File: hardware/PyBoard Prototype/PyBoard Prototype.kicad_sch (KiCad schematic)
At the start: 10 parts, among them J1 MIDI In, J2 MIDI Out, Q1 Q_PNP_BCE, U1 PyBoard_v1.1, U2 PC817, U3 MIKROE-506

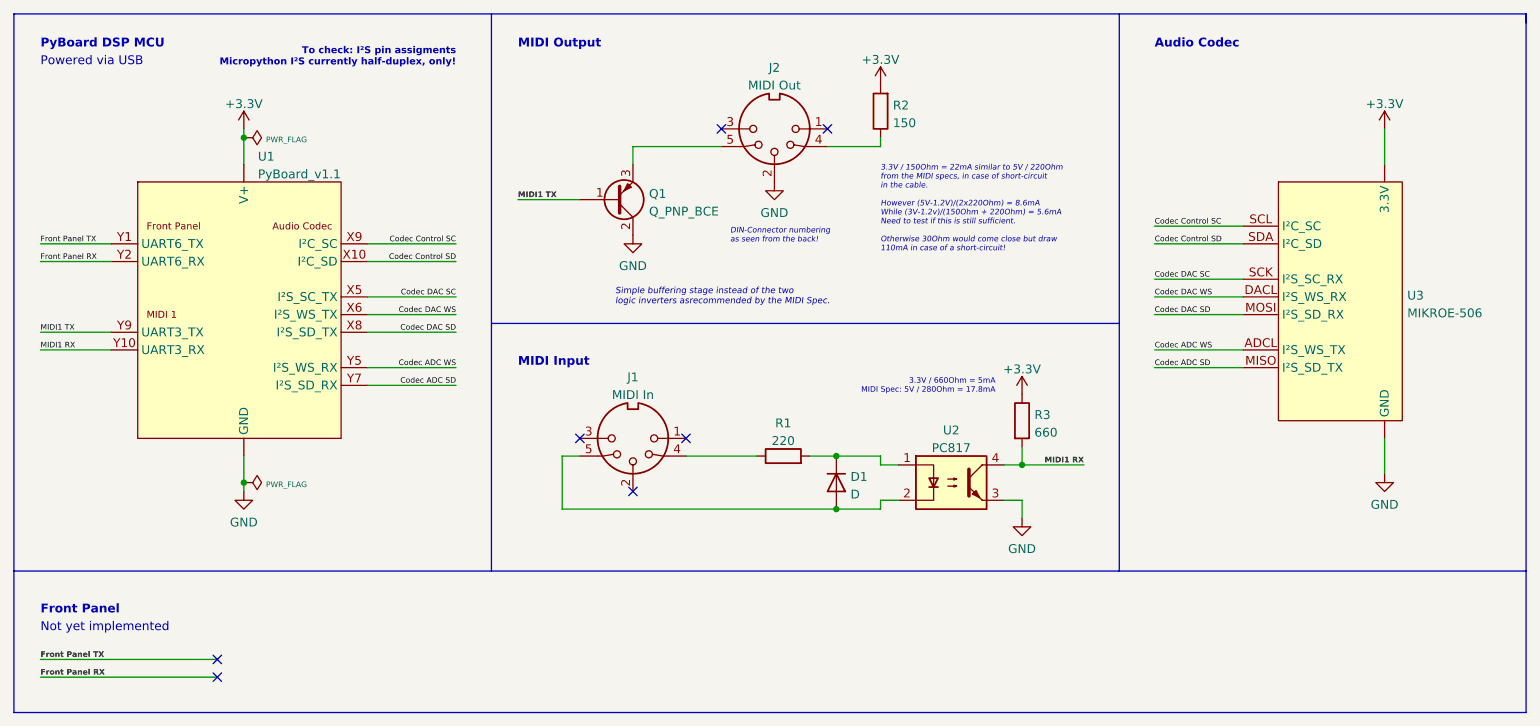
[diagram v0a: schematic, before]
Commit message: Some more experiments with MicroPython
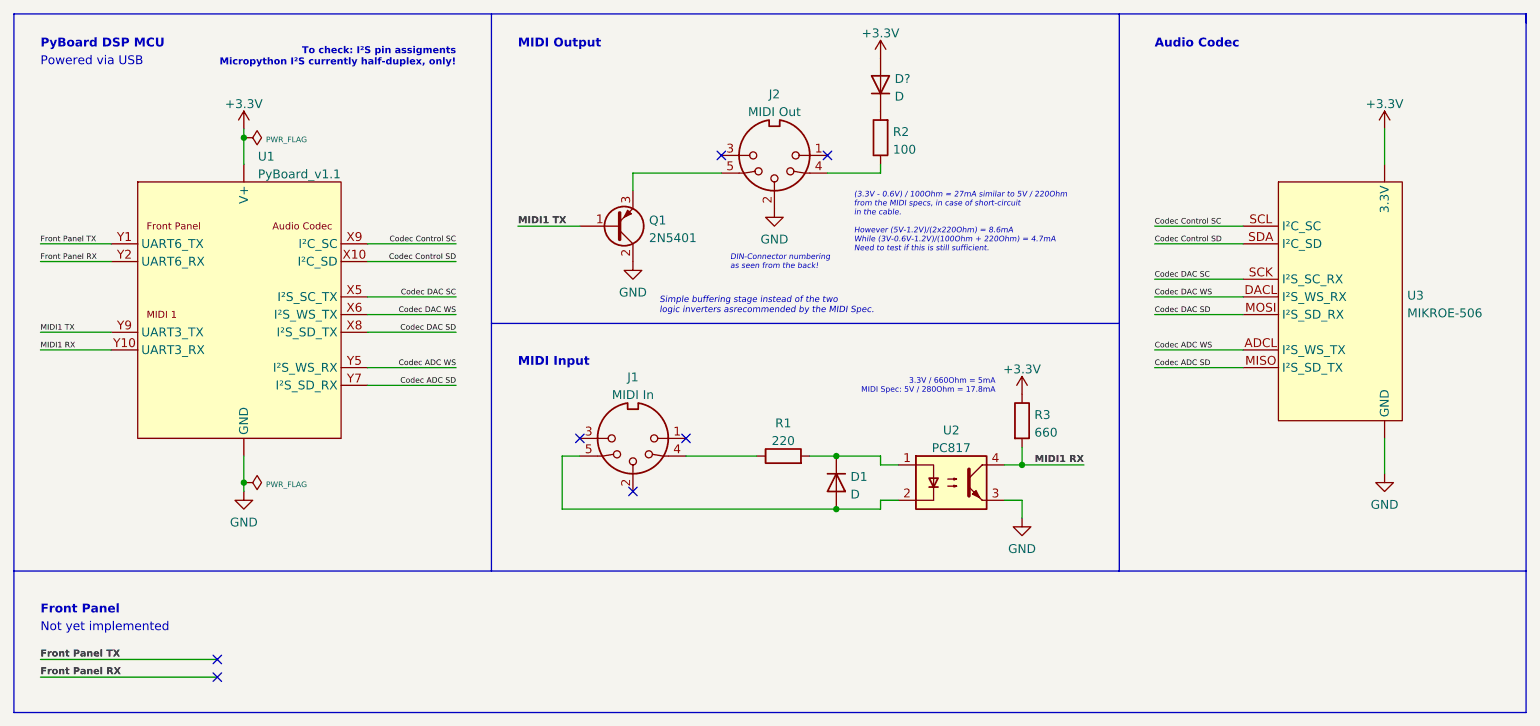
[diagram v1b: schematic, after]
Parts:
- added D?: D, symbol Device:D
- Q1: value Q_PNP_BCE -> 2N5401
- R2: value 150 -> 100
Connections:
- net +3V3: now also D?.2 (A); no longer R2.2
- new net: D?.1 (K), R2.2
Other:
- note added: "(3.3V - 0.6V) / 100Ohm = 27mA similar to 5V / 220Ohm from the MIDI specs, in case of short-circuit in the cable. However (5V-1.2V)/(2x220Ohm) = 8.6mA While (3V-0.6V-1.2V)/(100Ohm + 220Ohm) = 4.7mA Need to test if this is still sufficient."
- note removed: "3.3V / 150Ohm = 22mA similar to 5V / 220Ohm from the MIDI specs, in case of short-circuit in the cable. However (5V-1.2V)/(2x220Ohm) = 8.6mA While (3V-1.2v)/(150Ohm + 220Ohm) = 5.6mA Need to test if this is still sufficient. Otherwise 30Ohm would come close but draw 110mA in case of a short-circuit!"
- moved on the sheet: J2, Q1, R2
